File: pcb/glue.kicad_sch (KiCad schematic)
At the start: 60 parts, among them SW1 Opts, SW2 Reset Vector, SW3 NMI, SW4 RESET, U10 GAL16V8, U12 MCP100-475D, U2 74LS573, U3 74LS573, U4 74LS245, U5 74LS245, U6 74AHC273, U7 74LS240, U8 74LS240, U9 74LS259

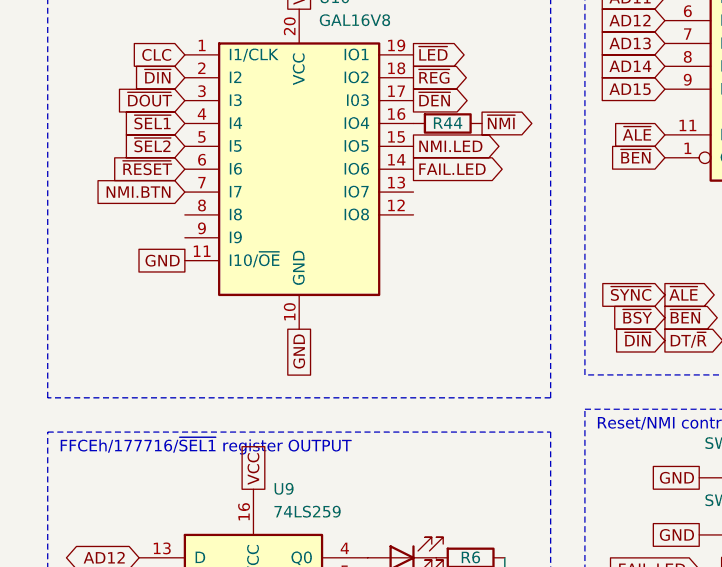
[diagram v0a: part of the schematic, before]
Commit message: final logic, gal, 3D
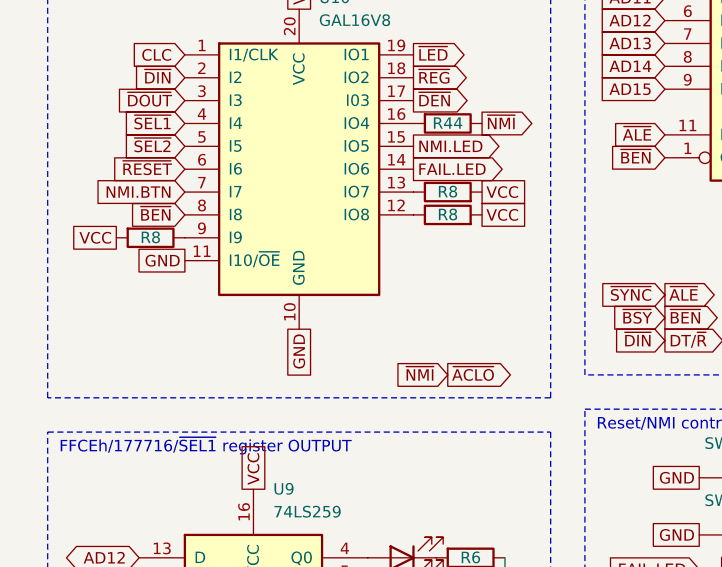
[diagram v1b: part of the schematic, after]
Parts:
- added R8 (x3): 0R, Resistor_SMD:R_0603_1608Metric_Pad0.98x0.95mm_HandSolder, symbol Device:R
- U10: footprint Package_DIP:DIP-20_W7.62mm -> Package_LCC:PLCC-20
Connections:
- net ~{NMI} is gone; now on net ~{ACLO}: R44.1, R6.1, U6.3 (D0)
- net VCC: now also R8.2, R8.2, R8.2
- net ~{BEN}: now also U10.8 (I8)
- net at U10.12 (IO8): now also R8.1
- net at U10.13 (IO7): now also R8.1
- net at U10.9 (I9): now also R8.1
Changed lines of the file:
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@@
+    )
+  )
+  (global_label "VCC" (shape passive) (at 74.93 118.11 0) (fields_autoplaced)
+    (effects (font (size 1.27 1.27)) (justify left))
+    (property "Intersheetrefs" "${INTERSHEET_REFS}" (at 80.4325 118.11 0)
+      (effects (font (size 1.27 1.27)) (justify left) hide)
     )
   )
@@
     )
   )
+  (global_label "VCC" (shape passive) (at 34.29 120.65 180) (fields_autoplaced)
+    (effects (font (size 1.27 1.27)) (justify right))
+    (property "Intersheetrefs" "${INTERSHEET_REFS}" (at 28.7875 120.65 0)
+      (effects (font (size 1.27 1.27)) (justify right) hide)
+    )
+  )
   (global_label "~{IRQ2}" (shape output) (at 67.31 39.37 0) (fields_autoplaced)
     (effects (font (size 1.27 1.27)) (justify left))
@@
     )
   )
+  (global_label "~{NMI}" (shape input) (at 71.12 135.89 180) (fields_autoplaced)
+    (effects (font (size 1.27 1.27)) (justify right))
+    (property "Intersheetrefs" "${INTERSHEET_REFS}" (at 64.7481 135.89 0)
+      (effects (font (size 1.27 1.27)) (justify right) hide)
+    )
+  )
   (global_label "VCC" (shape passive) (at 107.95 78.74 90) (fields_autoplaced)
     (effects (font (size 1.27 1.27)) (justify left))
@@
     )
   )
+  (global_label "~{ACLO}" (shape output) (at 71.12 135.89 0) (fields_autoplaced)
+    (effects (font (size 1.27 1.27)) (justify left))
+    (property "Intersheetrefs" "${INTERSHEET_REFS}" (at 78.8224 135.89 0)
+      (effects (font (size 1.27 1.27)) (justify left) hide)
+    )
+  )
   (global_label "AD9" (shape input) (at 95.25 88.9 180) (fields_autoplaced)
     (effects (font (size 1.27 1.27)) (justify right))
@@
     )
   )
+  (global_label "VCC" (shape passive) (at 74.93 115.57 0) (fields_autoplaced)
+    (effects (font (size 1.27 1.27)) (justify left))
+    (property "Intersheetrefs" "${INTERSHEET_REFS}" (at 80.4325 115.57 0)
+      (effects (font (size 1.27 1.27)) (justify left) hide)
+    )
+  )
   (global_label "~{ALE}" (shape input) (at 95.25 57.15 180) (fields_autoplaced)
     (effects (font (size 1.27 1.27)) (justify right))
@@
     (effects (font (size 1.27 1.27)) (justify right))
     (property "Intersheetrefs" "${INTERSHEET_REFS}" (at 179.6756 53.34 0)
+      (effects (font (size 1.27 1.27)) (justify right) hide)
+    )
+  )
+  (global_label "~{BEN}" (shape input) (at 41.91 118.11 180) (fields_autoplaced)
+    (effects (font (size 1.27 1.27)) (justify right))
+    (property "Intersheetrefs" "${INTERSHEET_REFS}" (at 35.1753 118.11 0)
       (effects (font (size 1.27 1.27)) (justify right) hide)
     )
@@
       (effects (font (size 1.27 1.27)) (justify left))
     )
-    (property "Footprint" "Package_DIP:DIP-20_W7.62mm" (at 54.61 113.03 0)
+    (property "Footprint" "Package_LCC:PLCC-20" (at 54.61 113.03 0)
       (effects (font (size 1.27 1.27)) hide)
     )
@@
     )
   )
+  (symbol (lib_id "Device:R") (at 38.1 120.65 270) (unit 1)
+    (in_bom yes) (on_board yes) (dnp no)
+    (property "Reference" "R8" (at 38.1 120.65 90)
+      (effects (font (size 1.27 1.27)))
+    )
+    (property "Value" "0R" (at 38.1 116.84 90)
+      (effects (font (size 1.27 1.27)) hide)
+    )
+    (property "Footprint" "Resistor_SMD:R_0603_1608Metric_Pad0.98x0.95mm_HandSolder" (at 38.1 118.872 90)
+      (effects (font (size 1.27 1.27)) hide)
+    )
+    (property "Datasheet" "~" (at 38.1 120.65 0)
+      (effects (font (size 1.27 1.27)) hide)
+    )
+    (pin "1")
+    (pin "2")
+    (instances
+      (project "KR1801"
+        (path "/68e08f4a-84cb-4510-afcb-23087110769d"
+          (reference "R8") (unit 1)
+        )
+        (path "/68e08f4a-84cb-4510-afcb-23087110769d/5a51aeec-6dcc-4755-ba2c-62e21ea48109"
+          (reference "R47") (unit 1)
+        )
+      )
+    )
+  )
+  (symbol (lib_id "Device:R") (at 71.12 115.57 90) (unit 1)
+    (in_bom yes) (on_board yes) (dnp no)
+    (property "Reference" "R8" (at 71.12 115.57 90)
+      (effects (font (size 1.27 1.27)))
+    )
+    (property "Value" "0R" (at 71.12 119.38 90)
+      (effects (font (size 1.27 1.27)) hide)
+    )
+    (property "Footprint" "Resistor_SMD:R_0603_1608Metric_Pad0.98x0.95mm_HandSolder" (at 71.12 117.348 90)
+      (effects (font (size 1.27 1.27)) hide)
+    )
+    (property "Datasheet" "~" (at 71.12 115.57 0)
+      (effects (font (size 1.27 1.27)) hide)
+    )
+    (pin "1")
+    (pin "2")
+    (instances
+      (project "KR1801"
+        (path "/68e08f4a-84cb-4510-afcb-23087110769d"
+          (reference "R8") (unit 1)
+        )
+        (path "/68e08f4a-84cb-4510-afcb-23087110769d/5a51aeec-6dcc-4755-ba2c-62e21ea48109"
+          (reference "R48") (unit 1)
+        )
+      )
+    )
+  )
   (symbol (lib_id "Device:R") (at 38.1 41.91 270) (unit 1)
     (in_bom yes) (on_board yes) (dnp no)
@@
         )
       )
+    )
+  )
+  (symbol (lib_id "Device:R") (at 71.12 118.11 90) (unit 1)
+    (in_bom yes) (on_board yes) (dnp no)
+    (property "Reference" "R8" (at 71.12 118.11 90)
+      (effects (font (size 1.27 1.27)))
+    )
+    (property "Value" "0R" (at 71.12 121.92 90)
+      (effects (font (size 1.27 1.27)) hide)
+    )
+    (property "Footprint" "Resistor_SMD:R_0603_1608Metric_Pad0.98x0.95mm_HandSolder" (at 71.12 119.888 90)
+      (effects (font (size 1.27 1.27)) hide)
+    )
+    (property "Datasheet" "~" (at 71.12 118.11 0)
+      (effects (font (size 1.27 1.27)) hide)
+    )
+    (pin "1")
+    (pin "2")
+    (instances
+      (project "KR1801"
+        (path "/68e08f4a-84cb-4510-afcb-23087110769d"
+          (reference "R8") (unit 1)
+        )
+        (path "/68e08f4a-84cb-4510-afcb-23087110769d/5a51aeec-6dcc-4755-ba2c-62e21ea48109"
+          (reference "R49") (unit 1)
+        )
+      )

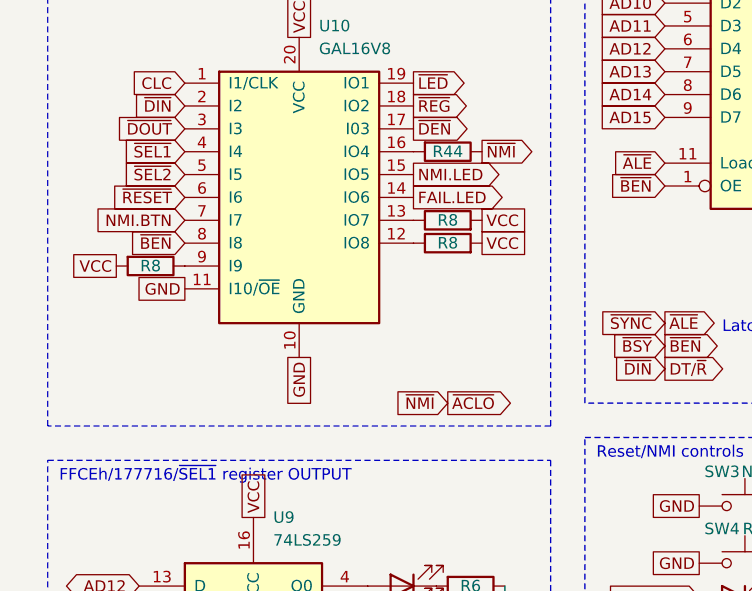
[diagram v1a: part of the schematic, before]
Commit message: /init
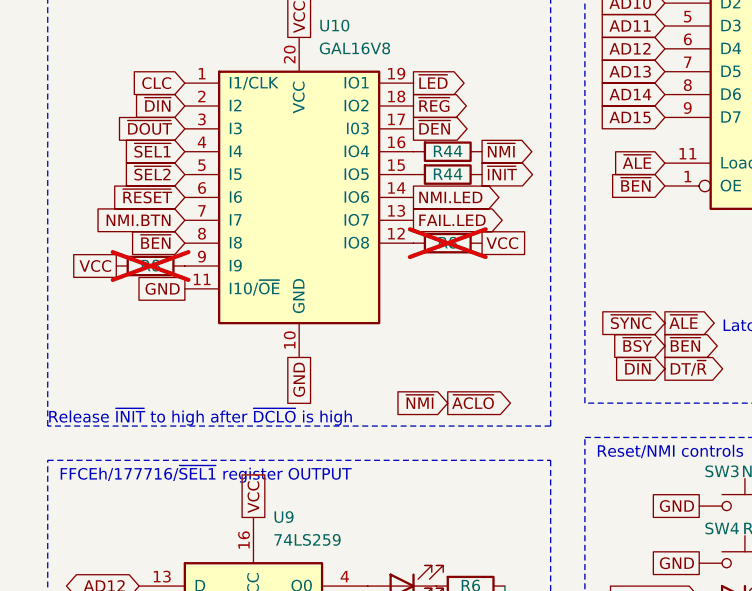
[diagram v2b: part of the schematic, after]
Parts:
- removed R8: 0R, Resistor_SMD:R_0603_1608Metric_Pad0.98x0.95mm_HandSolder, symbol Device:R
- added R44: 0R, Resistor_SMD:R_0603_1608Metric_Pad0.98x0.95mm_HandSolder, symbol Device:R
- R44: value NPR -> 0R
- R8: now not fitted
- R8: now not fitted; now left out of the parts list
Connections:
- net FAIL.LED: now also U10.13 (IO7); no longer U10.14 (IO6)
- net NMI.LED: now also U10.14 (IO6); no longer U10.15 (IO5)
- new net: R44.2, U10.15 (IO5)
- new net ~{INIT}: R44.1
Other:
- note added: "Release ~{INIT} to high after ~{DCLO} is high"
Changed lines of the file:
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@@
     (effects (font (size 1.27 1.27)) (justify left bottom))
   )
+  (text "Release ~{INIT} to high after ~{DCLO} is high" (at 26.67 138.43 0)
+    (effects (font (size 1.27 1.27)) (justify left bottom))
+  )
   (label "DR10" (at 201.93 90.17 0) (fields_autoplaced)
     (effects (font (size 1.27 1.27)) (justify left bottom))
@@
     )
   )
+  (global_label "NMI.LED" (shape output) (at 67.31 113.03 0) (fields_autoplaced)
+    (effects (font (size 1.27 1.27)) (justify left))
+    (property "Intersheetrefs" "${INTERSHEET_REFS}" (at 77.7338 113.03 0)
+      (effects (font (size 1.27 1.27)) (justify left) hide)
+    )
+  )
   (global_label "GND" (shape passive) (at 185.42 105.41 180) (fields_autoplaced)
     (effects (font (size 1.27 1.27)) (justify right))
@@
     )
   )
-  (global_label "NMI.LED" (shape output) (at 67.31 110.49 0) (fields_autoplaced)
-    (effects (font (size 1.27 1.27)) (justify left))
-    (property "Intersheetrefs" "${INTERSHEET_REFS}" (at 77.7338 110.49 0)
-      (effects (font (size 1.27 1.27)) (justify left) hide)
-    )
-  )
   (global_label "AD3" (shape input) (at 95.25 41.91 180) (fields_autoplaced)
     (effects (font (size 1.27 1.27)) (justify right))
@@
     )
   )
-  (global_label "FAIL.LED" (shape output) (at 67.31 113.03 0) (fields_autoplaced)
-    (effects (font (size 1.27 1.27)) (justify left))
-    (property "Intersheetrefs" "${INTERSHEET_REFS}" (at 78.1572 113.03 0)
-      (effects (font (size 1.27 1.27)) (justify left) hide)
-    )
-  )
   (global_label "GND" (shape passive) (at 99.06 147.32 180) (fields_autoplaced)
     (effects (font (size 1.27 1.27)) (justify right))
@@
     )
   )
+  (global_label "FAIL.LED" (shape output) (at 67.31 115.57 0) (fields_autoplaced)
+    (effects (font (size 1.27 1.27)) (justify left))
+    (property "Intersheetrefs" "${INTERSHEET_REFS}" (at 78.1572 115.57 0)
+      (effects (font (size 1.27 1.27)) (justify left) hide)
+    )
+  )
   (global_label "~{IRQ1}" (shape output) (at 67.31 36.83 0) (fields_autoplaced)
     (effects (font (size 1.27 1.27)) (justify left))
@@
     )
   )
+  (global_label "~{INIT}" (shape output) (at 74.93 110.49 0) (fields_autoplaced)
+    (effects (font (size 1.27 1.27)) (justify left))
+    (property "Intersheetrefs" "${INTERSHEET_REFS}" (at 81.4229 110.49 0)
+      (effects (font (size 1.27 1.27)) (justify left) hide)
+    )
+  )
   (global_label "VCC" (shape passive) (at 185.42 119.38 180) (fields_autoplaced)
     (effects (font (size 1.27 1.27)) (justify right))
@@
     )
   )
-  (global_label "VCC" (shape passive) (at 74.93 115.57 0) (fields_autoplaced)
-    (effects (font (size 1.27 1.27)) (justify left))
-    (property "Intersheetrefs" "${INTERSHEET_REFS}" (at 80.4325 115.57 0)
-      (effects (font (size 1.27 1.27)) (justify left) hide)
-    )
-  )
   (global_label "~{ALE}" (shape input) (at 95.25 57.15 180) (fields_autoplaced)
     (effects (font (size 1.27 1.27)) (justify right))
@@
       (effects (font (size 1.27 1.27)))
     )
-    (property "Value" "NPR" (at 71.12 104.14 90)
+    (property "Value" "0R" (at 71.12 104.14 90)
       (effects (font (size 1.27 1.27)) hide)
     )
@@
   )
   (symbol (lib_id "Device:R") (at 38.1 120.65 270) (unit 1)
-    (in_bom yes) (on_board yes) (dnp no)
+    (in_bom yes) (on_board no) (dnp yes)
     (property "Reference" "R8" (at 38.1 120.65 90)
       (effects (font (size 1.27 1.27)))
@@
     )
   )
-  (symbol (lib_id "Device:R") (at 71.12 115.57 90) (unit 1)
-    (in_bom yes) (on_board yes) (dnp no)
-    (property "Reference" "R8" (at 71.12 115.57 90)
-      (effects (font (size 1.27 1.27)))
-    )
-    (property "Value" "0R" (at 71.12 119.38 90)
-      (effects (font (size 1.27 1.27)) hide)
-    )
-    (property "Footprint" "Resistor_SMD:R_0603_1608Metric_Pad0.98x0.95mm_HandSolder" (at 71.12 117.348 90)
-      (effects (font (size 1.27 1.27)) hide)
-    )
-    (property "Datasheet" "~" (at 71.12 115.57 0)
-      (effects (font (size 1.27 1.27)) hide)
-    )
-    (pin "1")
-    (pin "2")
-    (instances
-      (project "KR1801"
-        (path "/68e08f4a-84cb-4510-afcb-23087110769d"
-          (reference "R8") (unit 1)
-        )
-        (path "/68e08f4a-84cb-4510-afcb-23087110769d/5a51aeec-6dcc-4755-ba2c-62e21ea48109"
-          (reference "R48") (unit 1)
-        )
-      )
-    )
-  )
   (symbol (lib_id "Device:R") (at 38.1 41.91 270) (unit 1)
     (in_bom yes) (on_board yes) (dnp no)
@@
     )
   )
+  (symbol (lib_id "Device:R") (at 71.12 110.49 270) (unit 1)
+    (in_bom yes) (on_board yes) (dnp no)
+    (property "Reference" "R44" (at 71.12 110.49 90)
+      (effects (font (size 1.27 1.27)))
+    )
+    (property "Value" "0R" (at 71.12 106.68 90)
+      (effects (font (size 1.27 1.27)) hide)
+    )
+    (property "Footprint" "Resistor_SMD:R_0603_1608Metric_Pad0.98x0.95mm_HandSolder" (at 71.12 108.712 90)
+      (effects (font (size 1.27 1.27)) hide)
+    )
+    (property "Datasheet" "~" (at 71.12 110.49 0)
+      (effects (font (size 1.27 1.27)) hide)
+    )
+    (pin "1")
+    (pin "2")
+    (instances
+      (project "KR1801"
+        (path "/68e08f4a-84cb-4510-afcb-23087110769d"
+          (reference "R44") (unit 1)
+        )
+        (path "/68e08f4a-84cb-4510-afcb-23087110769d/5a51aeec-6dcc-4755-ba2c-62e21ea48109"
+          (reference "R48") (unit 1)
+        )
+      )
+    )
+  )
   (symbol (lib_id "Switch:SW_DIP_x08") (at 194.31 43.18 0) (unit 1)
     (in_bom yes) (on_board yes) (dnp no) (fields_autoplaced)
@@
   )
   (symbol (lib_id "Device:R") (at 71.12 118.11 90) (unit 1)
-    (in_bom yes) (on_board yes) (dnp no)
+    (in_bom no) (on_board yes) (dnp yes)
     (property "Reference" "R8" (at 71.12 118.11 90)
       (effects (font (size 1.27 1.27)))
